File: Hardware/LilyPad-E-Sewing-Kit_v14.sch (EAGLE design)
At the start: 51 parts

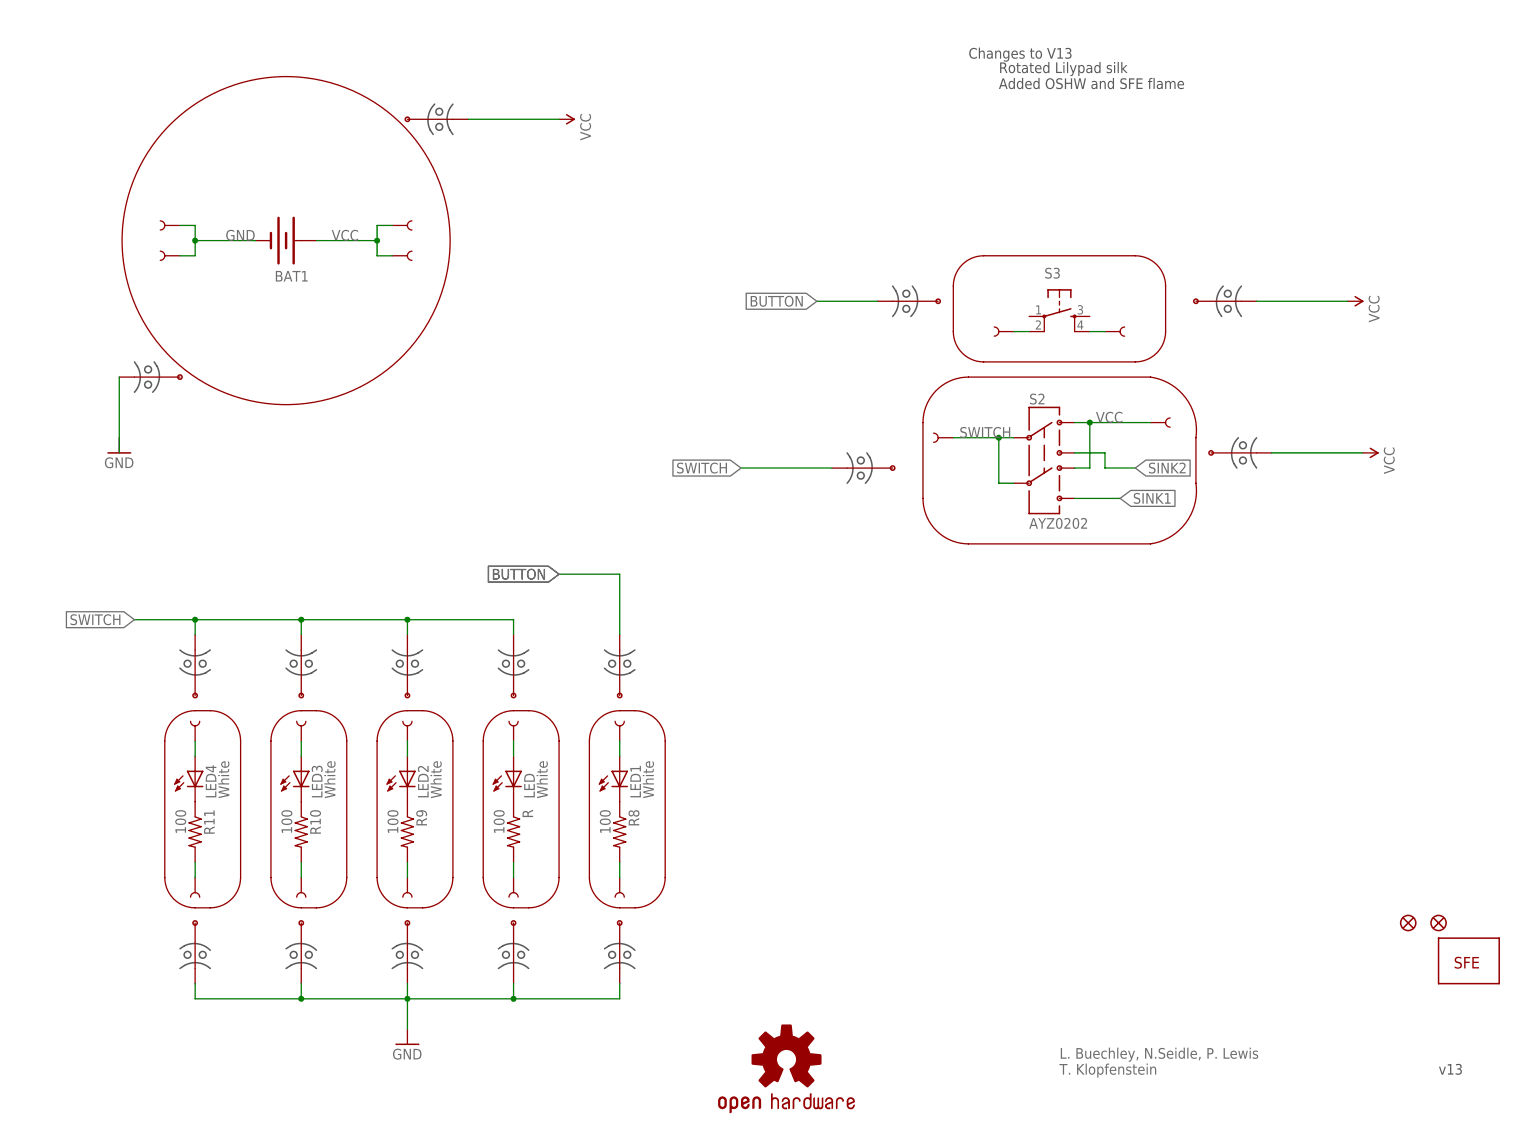
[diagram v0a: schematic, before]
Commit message: Updated files
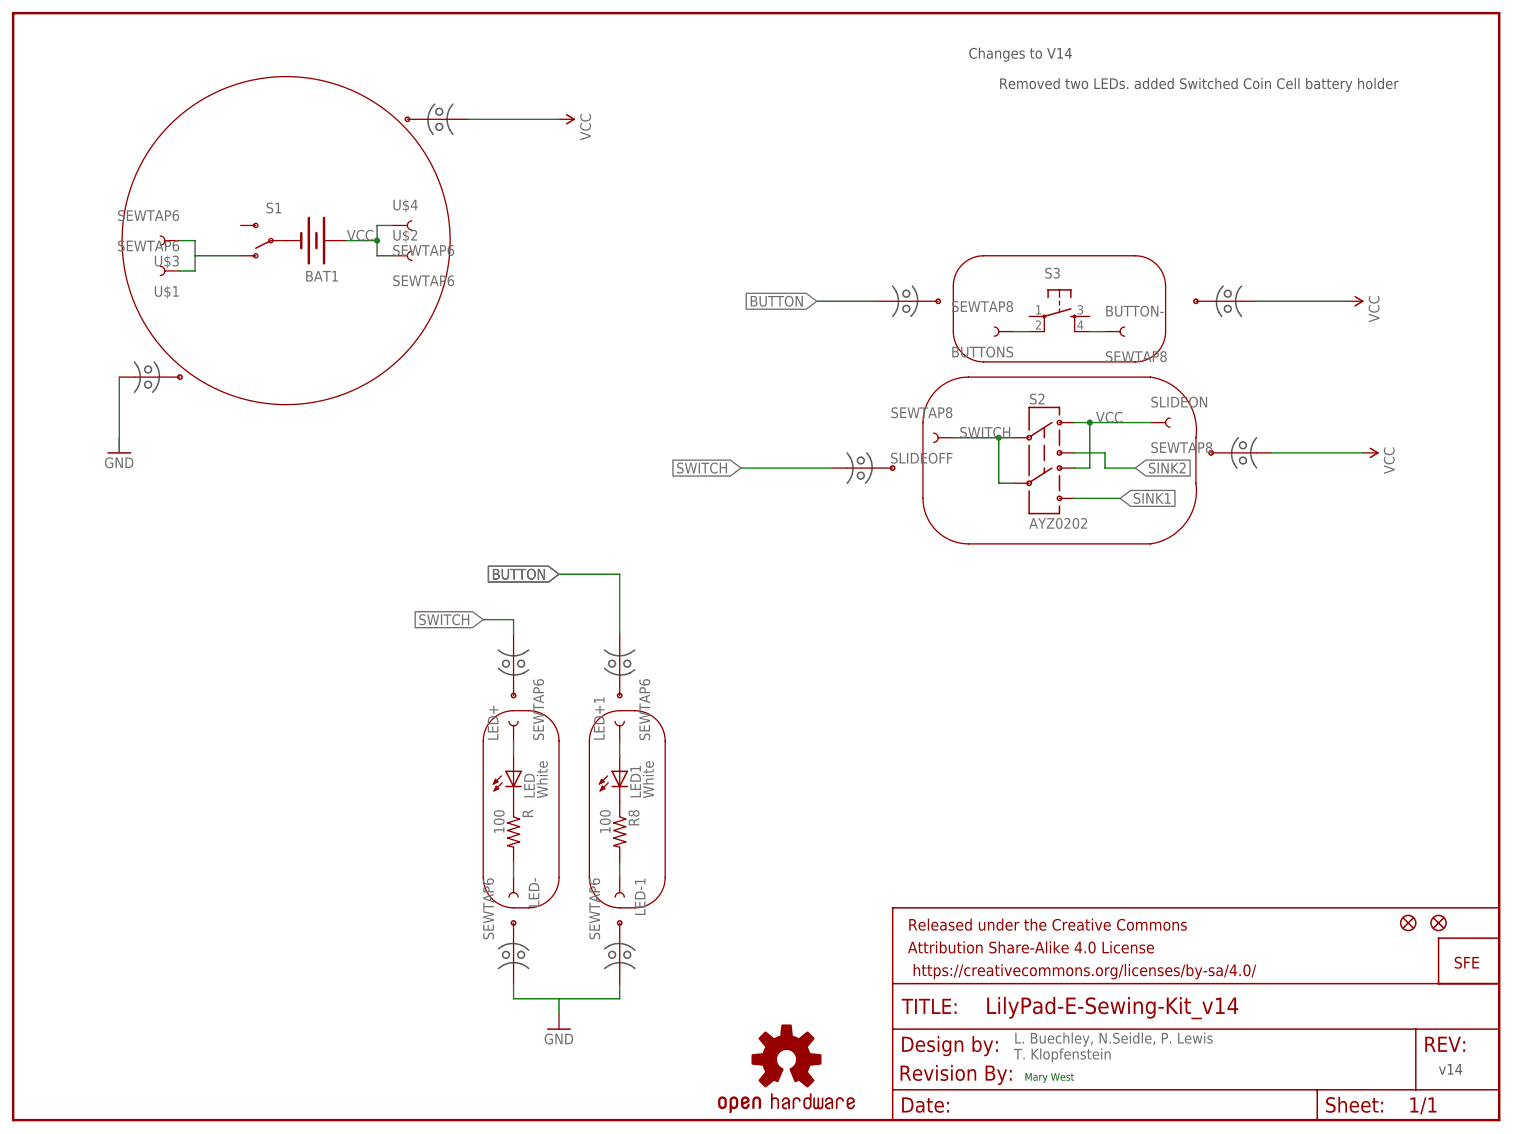
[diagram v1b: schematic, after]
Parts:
- removed LED+2, LED+3, LED+4, LED-2, LED-3, LED-4: SEWTAP6, LilyPad-Wearables:SEWTAP6
- removed LED2, LED3, LED4: White, SparkFun-3-2-07:LED1206
- removed R10, R11, R9: 100, SparkFun:RESISTOR0603-RES
- removed U$10, U$11, U$12, U$15, U$16, U$17: MOUSE-BITE-12_HOLES, Testing:MOUSE-BITE-12_HOLES
- added FRAME1: FRAME-LETTER, SparkFun-Aesthetics:FRAME-LETTER
- added S1: (no value), SparkFun-Electromechanical:SWITCH-SPDTSMD
- added U$5: REVISION, SparkFun-Aesthetics:REVISION
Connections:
- removed net N$24: LED2.C, R9.1
- removed net N$27: LED3.C, R10.1
- removed net N$30: LED4.C, R11.1
- new net N$1: BAT1.-, S1.P
- net GND: no longer BAT1.-, LED-2.1, LED-3.1, LED-4.1, R10.2, R11.2, R9.2, U$15.P$1, U$16.P$1, U$17.P$1
- net SWITCH: no longer LED+2.1, LED+3.1, LED+4.1, LED2.A, LED3.A, LED4.A, U$10.P$1, U$11.P$1, U$12.P$1
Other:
- note added: "Changes to V14"
- note added: "Mary West"
- note added: "Removed two LEDs. added Switched Coin Cell battery holder"
- note added: "v14"
- note removed: "Changes to V13"
- note removed: "Rotated Lilypad silk Added OSHW and SFE flame"
- note removed: "v13"
- moved on the sheet: BAT1
